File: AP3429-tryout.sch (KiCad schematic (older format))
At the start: 61 parts, among them J1 Conn_01x05, J2 Conn_01x02, U1 AP3429, U10 AMS1117-3.3, U2 AP3429, U3 AP3429, U4 AP2120N, U5 AMS1117-3.3, U6 AMS1117-3.3, U7 AMS1117-3.3, U8 AMS1117-3.3, U9 AMS1117-3.3

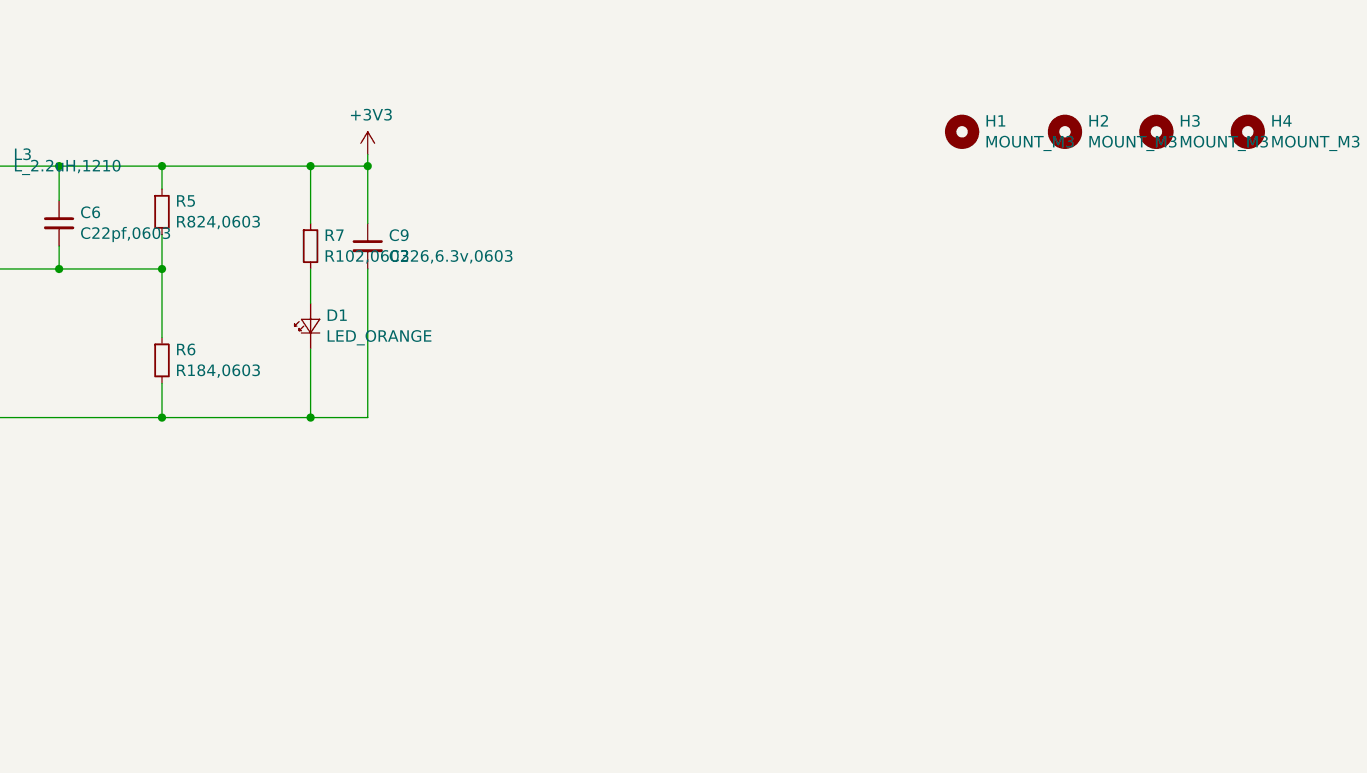
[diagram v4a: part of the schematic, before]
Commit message: update,
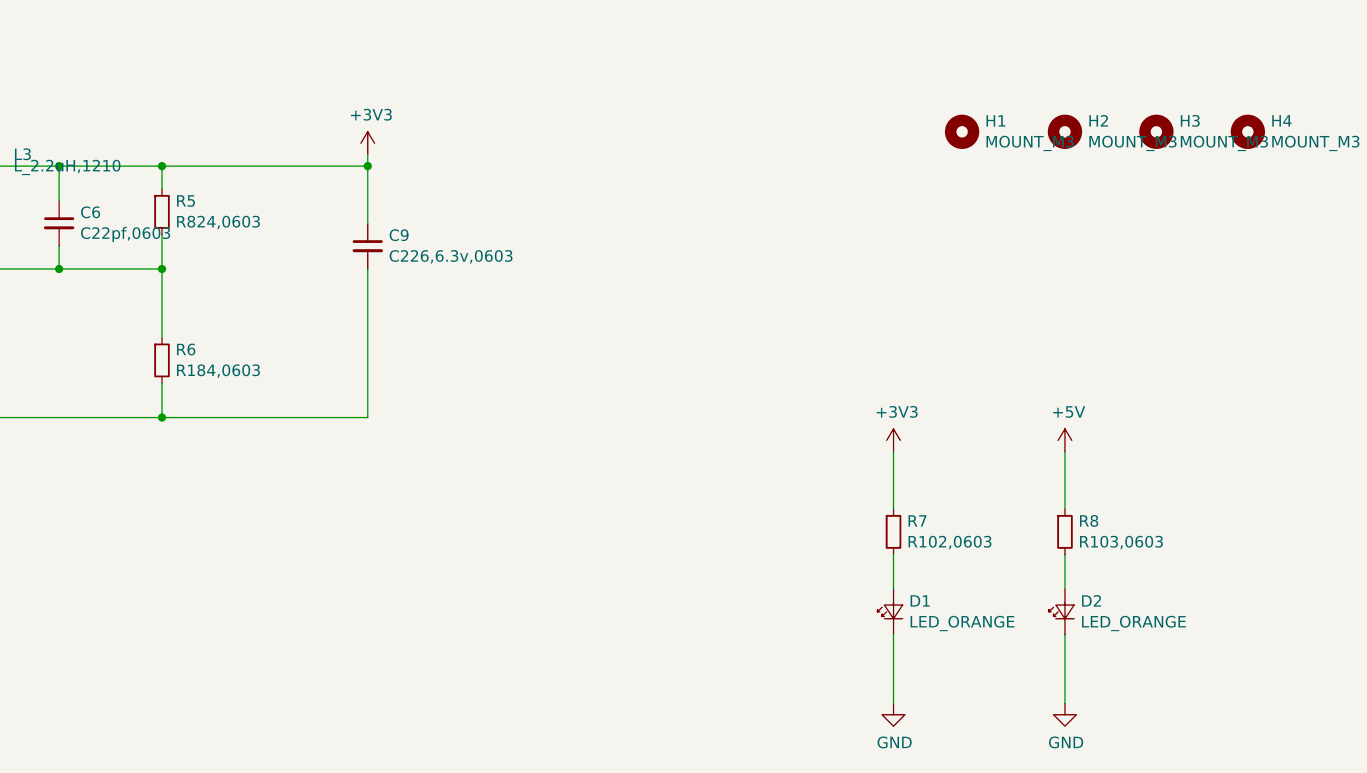
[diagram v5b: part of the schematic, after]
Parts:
- added D2: LED_ORANGE, LED_SMD:LED_0805_2012Metric_Castellated, symbol taobao-led:LED_ORANGE
- added R8: R103,0603, Resistor_SMD:R_0603_1608Metric_Pad1.05x0.95mm_HandSolder, symbol taobao-r:R103,0603
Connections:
- net +5V: now also R8.1
- net GND: now also D2.1 (K)
- new net: D2.2 (A), R8.2
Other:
- moved on the sheet: D1, R7
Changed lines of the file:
@@
 EELAYER 26 0
 EELAYER END
-$Descr A4 11693 8268
+$Descr A3 16535 11693
 encoding utf-8
 Sheet 1 1
@@
 Wire Wire Line
 	6500 5700 6500 5750
-Wire Wire Line
-	6500 5750 6250 5750
 Connection ~ 5600 5750
 Wire Wire Line
@@
 Wire Wire Line
 	6500 6200 6500 6850
-Wire Wire Line
-	6500 6850 6250 6850
 Connection ~ 5600 6850
 $Comp
@@
 L taobao-led:LED_ORANGE D1
 U 1 1 5C042628
-P 6250 6450
-F 0 "D1" V 6296 6382 50  0000 R CNN
-F 1 "LED_ORANGE" V 6205 6382 50  0000 R CNN
-F 2 "LED_SMD:LED_0805_2012Metric_Castellated" V 6250 6450 50  0001 C CNN
-F 3 "~" V 6250 6450 50  0001 C CNN
-	1    6250 6450
+P 8800 7700
+F 0 "D1" V 8846 7632 50  0000 R CNN
+F 1 "LED_ORANGE" V 8755 7632 50  0000 R CNN
+F 2 "LED_SMD:LED_0805_2012Metric_Castellated" V 8800 7700 50  0001 C CNN
+F 3 "~" V 8800 7700 50  0001 C CNN
+	1    8800 7700
 	0    -1   -1   0
 $EndComp
@@
 L taobao-r:R102,0603 R7
 U 1 1 5C04282E
-P 6250 6100
-F 0 "R7" H 6309 6146 50  0000 L CNN
-F 1 "R102,0603" H 6309 6055 50  0000 L CNN
-F 2 "Resistor_SMD:R_0603_1608Metric_Pad1.05x0.95mm_HandSolder" H 6250 6100 50  0001 C CNN
-F 3 "~" H 6250 6100 50  0001 C CNN
-	1    6250 6100
-	1    0    0    -1
-$EndComp
-Wire Wire Line
-	6250 6000 6250 5750
-Connection ~ 6250 5750
-Wire Wire Line
-	6250 5750 5600 5750
-Wire Wire Line
-	6250 6200 6250 6350
-Wire Wire Line
-	6250 6550 6250 6850
-Connection ~ 6250 6850
-Wire Wire Line
-	6250 6850 5600 6850
+P 8800 7350
+F 0 "R7" H 8859 7396 50  0000 L CNN
+F 1 "R102,0603" H 8859 7305 50  0000 L CNN
+F 2 "Resistor_SMD:R_0603_1608Metric_Pad1.05x0.95mm_HandSolder" H 8800 7350 50  0001 C CNN
+F 3 "~" H 8800 7350 50  0001 C CNN
+	1    8800 7350
+	1    0    0    -1
+$EndComp
+Wire Wire Line
+	8800 7250 8800 7000
+Wire Wire Line
+	8800 7450 8800 7600
+Wire Wire Line
+	8800 7800 8800 8100
 $Comp
 L power:+3V3 #PWR0110
@@
 	0    -1   -1   0
 $EndComp
+Wire Wire Line
+	5600 5750 6500 5750
+Wire Wire Line
+	5600 6850 6500 6850
+$Comp
+L power:+3V3 #PWR0132
+U 1 1 5C078F9C
+P 8800 7000
+F 0 "#PWR0132" H 8800 6850 50  0001 C CNN
+F 1 "+3V3" H 8815 7173 50  0000 C CNN
+F 2 "" H 8800 7000 50  0001 C CNN
+F 3 "" H 8800 7000 50  0001 C CNN
+	1    8800 7000
+	1    0    0    -1
+$EndComp
+$Comp
+L power:GND #PWR0133
+U 1 1 5C079499
+P 8800 8100
+F 0 "#PWR0133" H 8800 7850 50  0001 C CNN
+F 1 "GND" H 8805 7927 50  0000 C CNN
+F 2 "" H 8800 8100 50  0001 C CNN
+F 3 "" H 8800 8100 50  0001 C CNN
+	1    8800 8100
+	1    0    0    -1
+$EndComp
+$Comp
+L taobao-led:LED_ORANGE D2
+U 1 1 5C079972
+P 9550 7700
+F 0 "D2" V 9596 7632 50  0000 R CNN
+F 1 "LED_ORANGE" V 9505 7632 50  0000 R CNN
+F 2 "LED_SMD:LED_0805_2012Metric_Castellated" V 9550 7700 50  0001 C CNN
+F 3 "~" V 9550 7700 50  0001 C CNN
+	1    9550 7700
+	0    -1   -1   0
+$EndComp
+Wire Wire Line
+	9550 7250 9550 7000
+Wire Wire Line
+	9550 7450 9550 7600
+Wire Wire Line
+	9550 7800 9550 8100
+$Comp
+L power:GND #PWR0134
+U 1 1 5C079987
+P 9550 8100
+F 0 "#PWR0134" H 9550 7850 50  0001 C CNN
+F 1 "GND" H 9555 7927 50  0000 C CNN
+F 2 "" H 9550 8100 50  0001 C CNN
+F 3 "" H 9550 8100 50  0001 C CNN
+	1    9550 8100
+	1    0    0    -1
+$EndComp
+$Comp
+L power:+5V #PWR0135
+U 1 1 5C08342C
+P 9550 7000
+F 0 "#PWR0135" H 9550 6850 50  0001 C CNN
+F 1 "+5V" H 9565 7173 50  0000 C CNN
+F 2 "" H 9550 7000 50  0001 C CNN
+F 3 "" H 9550 7000 50  0001 C CNN
+	1    9550 7000
+	1    0    0    -1
+$EndComp
+$Comp
+L taobao-r:R103,0603 R8
+U 1 1 5C083A53
+P 9550 7350
+F 0 "R8" H 9609 7396 50  0000 L CNN
+F 1 "R103,0603" H 9609 7305 50  0000 L CNN
+F 2 "Resistor_SMD:R_0603_1608Metric_Pad1.05x0.95mm_HandSolder" H 9550 7350 50  0001 C CNN
+F 3 "~" H 9550 7350 50  0001 C CNN
+	1    9550 7350
+	1    0    0    -1
+$EndComp
 $EndSCHEMATC
